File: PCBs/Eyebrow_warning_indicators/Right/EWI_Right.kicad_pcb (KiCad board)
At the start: 2 copper layers, 96.1 x 78.8 mm, 43 parts, among them J1 Conn_01x02_Female, J2 Conn_01x06_Male, J3 Conn_01x08_Male, J4 Conn_01x02_Female, J5 Conn_01x02_Female, SW1 IN SWTCH, SW2 OUT SWTCH

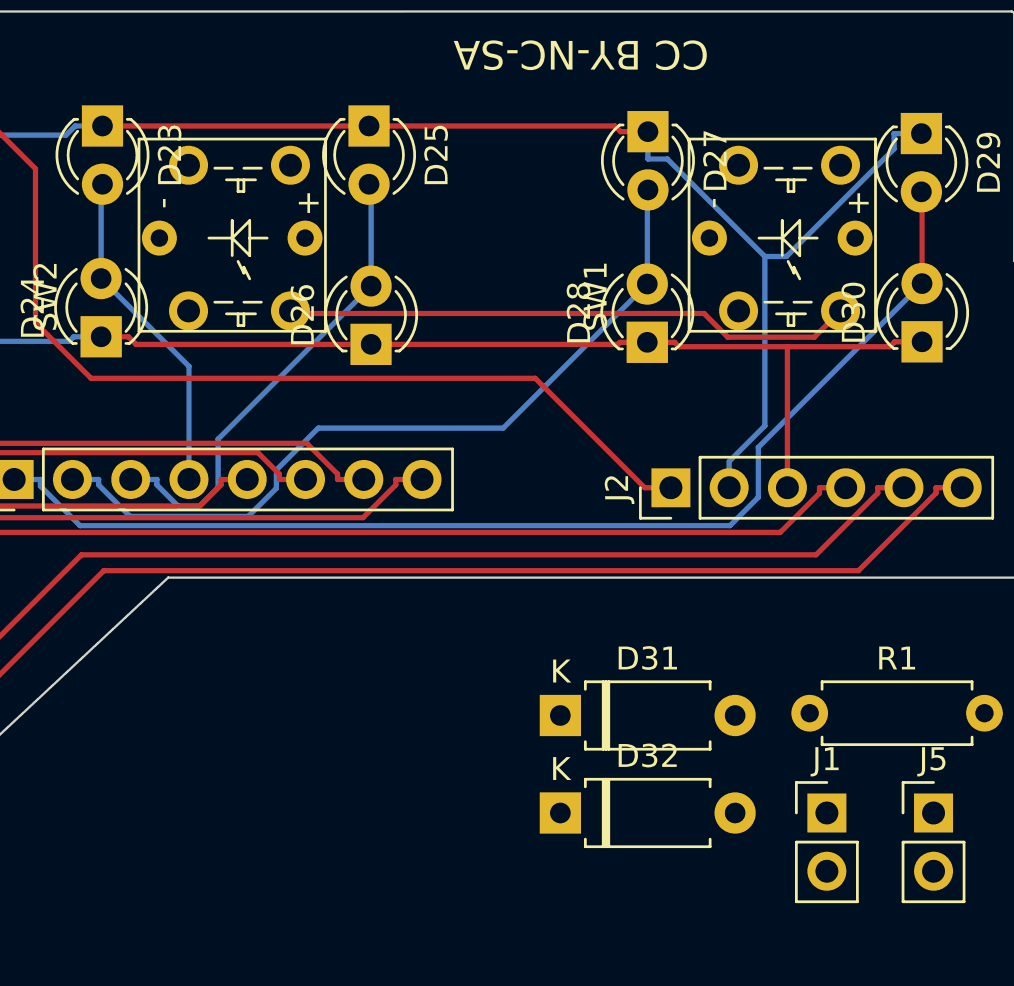
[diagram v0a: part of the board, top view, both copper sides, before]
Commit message: pcb
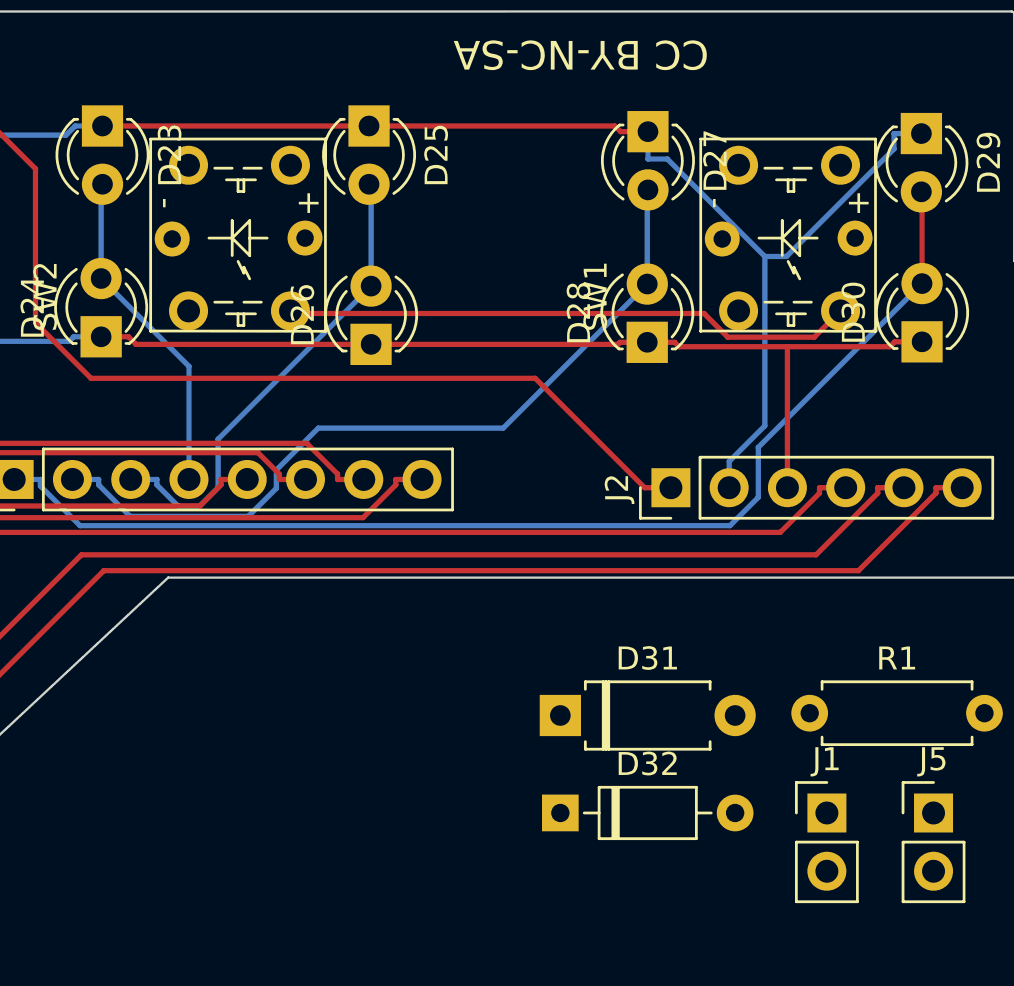
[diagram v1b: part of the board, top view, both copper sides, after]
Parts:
- D32: footprint Diode_THT:D_A-405_P7.62mm_Horizontal -> Diode_THT:D_DO-35_SOD27_P7.62mm_Horizontal
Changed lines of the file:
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@@
     (uvia_drill 0.1)
+  )
+  (module Diode_THT:D_DO-35_SOD27_P7.62mm_Horizontal (layer F.Cu)
+    (at 196.34 79.83)
+    (descr "Diode, DO-35_SOD27 series, Axial, Horizontal, pin pitch=7.62mm, , length*diameter=4*2mm^2, , http://www.diodes.com/_files/packages/DO-35.pdf")
+    (tags "Diode DO-35_SOD27 series Axial Horizontal pin pitch 7.62mm  length 4mm diameter 2mm")
+    (fp_text reference D32 (at 3.81 -2.12) (layer F.SilkS)
+      (effects (font (size 1 1) (thickness 0.15)))
+    )
+    (fp_text value D (at 3.81 2.12) (layer F.Fab)
+      (effects (font (size 1 1) (thickness 0.15)))
+    )
+    (fp_text user K (at 0 -1.8) (layer F.Fab)
+      (effects (font (size 1 1) (thickness 0.15)))
+    )
+    (fp_text user K (at 0 -1.8) (layer F.Fab)
+      (effects (font (size 1 1) (thickness 0.15)))
+    )
+    (fp_text user %R (at 4.11 0) (layer F.Fab)
+      (effects (font (size 0.8 0.8) (thickness 0.12)))
+    )
+    (fp_line (start 8.67 -1.25) (end -1.05 -1.25) (layer F.CrtYd) (width 0.05))
+    (fp_line (start 8.67 1.25) (end 8.67 -1.25) (layer F.CrtYd) (width 0.05))
+    (fp_line (start -1.05 1.25) (end 8.67 1.25) (layer F.CrtYd) (width 0.05))
+    (fp_line (start -1.05 -1.25) (end -1.05 1.25) (layer F.CrtYd) (width 0.05))
+    (fp_line (start 2.29 -1.12) (end 2.29 1.12) (layer F.SilkS) (width 0.12))
+    (fp_line (start 2.53 -1.12) (end 2.53 1.12) (layer F.SilkS) (width 0.12))
+    (fp_line (start 2.41 -1.12) (end 2.41 1.12) (layer F.SilkS) (width 0.12))
+    (fp_line (start 6.58 0) (end 5.93 0) (layer F.SilkS) (width 0.12))
+    (fp_line (start 1.04 0) (end 1.69 0) (layer F.SilkS) (width 0.12))
+    (fp_line (start 5.93 -1.12) (end 1.69 -1.12) (layer F.SilkS) (width 0.12))
+    (fp_line (start 5.93 1.12) (end 5.93 -1.12) (layer F.SilkS) (width 0.12))
+    (fp_line (start 1.69 1.12) (end 5.93 1.12) (layer F.SilkS) (width 0.12))
+    (fp_line (start 1.69 -1.12) (end 1.69 1.12) (layer F.SilkS) (width 0.12))
+    (fp_line (start 2.31 -1) (end 2.31 1) (layer F.Fab) (width 0.1))
+    (fp_line (start 2.51 -1) (end 2.51 1) (layer F.Fab) (width 0.1))
+    (fp_line (start 2.41 -1) (end 2.41 1) (layer F.Fab) (width 0.1))
+    (fp_line (start 7.62 0) (end 5.81 0) (layer F.Fab) (width 0.1))
+    (fp_line (start 0 0) (end 1.81 0) (layer F.Fab) (width 0.1))
+    (fp_line (start 5.81 -1) (end 1.81 -1) (layer F.Fab) (width 0.1))
+    (fp_line (start 5.81 1) (end 5.81 -1) (layer F.Fab) (width 0.1))
+    (fp_line (start 1.81 1) (end 5.81 1) (layer F.Fab) (width 0.1))
+    (fp_line (start 1.81 -1) (end 1.81 1) (layer F.Fab) (width 0.1))
+    (pad 2 thru_hole oval (at 7.62 0) (size 1.6 1.6) (drill 0.8) (layers *.Cu *.Mask)
+      (net 17 "Net-(D32-Pad2)"))
+    (pad 1 thru_hole rect (at 0 0) (size 1.6 1.6) (drill 0.8) (layers *.Cu *.Mask)
+      (net 18 "Net-(D32-Pad1)"))
+    (model ${KISYS3DMOD}/Diode_THT.3dshapes/D_DO-35_SOD27_P7.62mm_Horizontal.wrl
+      (at (xyz 0 0 0))
+      (scale (xyz 1 1 1))
+      (rotate (xyz 0 0 0))
+    )
   )
   (module Resistor_THT:R_Axial_DIN0207_L6.3mm_D2.5mm_P7.62mm_Horizontal (layer F.Cu)
@@
   )
   (module Diode_THT:D_A-405_P7.62mm_Horizontal (layer F.Cu)
-    (at 196.34 79.83)
-    (descr "Diode, A-405 series, Axial, Horizontal, pin pitch=7.62mm, , length*diameter=5.2*2.7mm^2, , http://www.diodes.com/_files/packages/A-405.pdf")
-    (tags "Diode A-405 series Axial Horizontal pin pitch 7.62mm  length 5.2mm diameter 2.7mm")
-    (fp_text reference D32 (at 3.81 -2.47) (layer F.SilkS)
-      (effects (font (size 1 1) (thickness 0.15)))
-    )
-    (fp_text value D (at 3.81 2.47) (layer F.Fab)
-      (effects (font (size 1 1) (thickness 0.15)))
-    )
-    (fp_text user K (at 0 -1.9) (layer F.SilkS)
-      (effects (font (size 1 1) (thickness 0.15)))
-    )
-    (fp_text user K (at 0 -1.9) (layer F.Fab)
-      (effects (font (size 1 1) (thickness 0.15)))
-    )
-    (fp_text user %R (at 4.2 0) (layer F.Fab)
-      (effects (font (size 1 1) (thickness 0.15)))
-    )
-    (fp_line (start 8.77 -1.6) (end -1.15 -1.6) (layer F.CrtYd) (width 0.05))
-    (fp_line (start 8.77 1.6) (end 8.77 -1.6) (layer F.CrtYd) (width 0.05))
-    (fp_line (start -1.15 1.6) (end 8.77 1.6) (layer F.CrtYd) (width 0.05))
-    (fp_line (start -1.15 -1.6) (end -1.15 1.6) (layer F.CrtYd) (width 0.05))
-    (fp_line (start 1.87 -1.47) (end 1.87 1.47) (layer F.SilkS) (width 0.12))
-    (fp_line (start 2.11 -1.47) (end 2.11 1.47) (layer F.SilkS) (width 0.12))
-    (fp_line (start 1.99 -1.47) (end 1.99 1.47) (layer F.SilkS) (width 0.12))
-    (fp_line (start 6.53 1.47) (end 6.53 1.14) (layer F.SilkS) (width 0.12))
-    (fp_line (start 1.09 1.47) (end 6.53 1.47) (layer F.SilkS) (width 0.12))
-    (fp_line (start 1.09 1.14) (end 1.09 1.47) (layer F.SilkS) (width 0.12))
-    (fp_line (start 6.53 -1.47) (end 6.53 -1.14) (layer F.SilkS) (width 0.12))
-    (fp_line (start 1.09 -1.47) (end 6.53 -1.47) (layer F.SilkS) (width 0.12))
-    (fp_line (start 1.09 -1.14) (end 1.09 -1.47) (layer F.SilkS) (width 0.12))
-    (fp_line (start 1.89 -1.35) (end 1.89 1.35) (layer F.Fab) (width 0.1))
-    (fp_line (start 2.09 -1.35) (end 2.09 1.35) (layer F.Fab) (width 0.1))
-    (fp_line (start 1.99 -1.35) (end 1.99 1.35) (layer F.Fab) (width 0.1))
-    (fp_line (start 7.62 0) (end 6.41 0) (layer F.Fab) (width 0.1))
-    (fp_line (start 0 0) (end 1.21 0) (layer F.Fab) (width 0.1))
-    (fp_line (start 6.41 -1.35) (end 1.21 -1.35) (layer F.Fab) (width 0.1))
-    (fp_line (start 6.41 1.35) (end 6.41 -1.35) (layer F.Fab) (width 0.1))
-    (fp_line (start 1.21 1.35) (end 6.41 1.35) (layer F.Fab) (width 0.1))
-    (fp_line (start 1.21 -1.35) (end 1.21 1.35) (layer F.Fab) (width 0.1))
-    (pad 2 thru_hole oval (at 7.62 0) (size 1.8 1.8) (drill 0.9) (layers *.Cu *.Mask)
-      (net 17 "Net-(D32-Pad2)"))
-    (pad 1 thru_hole rect (at 0 0) (size 1.8 1.8) (drill 0.9) (layers *.Cu *.Mask)
-      (net 18 "Net-(D32-Pad1)"))
-    (model ${KISYS3DMOD}/Diode_THT.3dshapes/D_A-405_P7.62mm_Horizontal.wrl
-      (at (xyz 0 0 0))
-      (scale (xyz 1 1 1))
-      (rotate (xyz 0 0 0))
-    )
-  )
-  (module Diode_THT:D_A-405_P7.62mm_Horizontal (layer F.Cu)
     (at 196.34 75.58)
     (descr "Diode, A-405 series, Axial, Horizontal, pin pitch=7.62mm, , length*diameter=5.2*2.7mm^2, , http://www.diodes.com/_files/packages/A-405.pdf")
@@
       (effects (font (size 1 1) (thickness 0.15)))
     )
-    (fp_text user K (at 0 -1.9) (layer F.SilkS)
+    (fp_text user K (at 0 -1.9) (layer F.Fab)
       (effects (font (size 1 1) (thickness 0.15)))
     )
@@
     )
     (fp_line (start -4.318 -3.81) (end -3.048 -3.81) (layer F.SilkS) (width 0.12))
-    (fp_line (start -4.318 4.318) (end -4.318 -3.81) (layer F.SilkS) (width 0.12))
-    (fp_line (start 4.064 4.318) (end -4.318 4.318) (layer F.SilkS) (width 0.12))
-    (fp_line (start 4.064 -3.81) (end 4.064 4.318) (layer F.SilkS) (width 0.12))
+    (fp_line (start -4.32 3.81) (end -4.318 -3.81) (layer F.SilkS) (width 0.12))
+    (fp_line (start 4.07 3.81) (end -4.312 3.81) (layer F.SilkS) (width 0.12))
+    (fp_line (start 4.064 -3.81) (end 4.05 3.81) (layer F.SilkS) (width 0.12))
     (fp_line (start -4.064 -3.81) (end 4.064 -3.81) (layer F.SilkS) (width 0.12))
     (fp_text user - (at -1.524 3.302 90) (layer F.SilkS)
@@
       (effects (font (size 1 1) (thickness 0.15)))
     )
-    (pad 6 thru_hole circle (at 0 3.429 270) (size 1.524 1.524) (drill 0.762) (layers *.Cu *.Mask)
+    (pad 6 thru_hole circle (at 0.04 2.87 270) (size 1.524 1.524) (drill 0.762) (layers *.Cu *.Mask)
       (net 19 "Net-(J1-Pad2)"))
     (pad 5 thru_hole circle (at 0 -2.921 270) (size 1.524 1.524) (drill 0.762) (layers *.Cu *.Mask)
@@
     )
     (fp_line (start -4.318 -3.81) (end -3.048 -3.81) (layer F.SilkS) (width 0.12))
-    (fp_line (start -4.318 4.318) (end -4.318 -3.81) (layer F.SilkS) (width 0.12))
-    (fp_line (start 4.064 4.318) (end -4.318 4.318) (layer F.SilkS) (width 0.12))
-    (fp_line (start 4.064 -3.81) (end 4.064 4.318) (layer F.SilkS) (width 0.12))
+    (fp_line (start -4.32 3.81) (end -4.318 -3.81) (layer F.SilkS) (width 0.12))
+    (fp_line (start 4.07 3.81) (end -4.312 3.81) (layer F.SilkS) (width 0.12))
+    (fp_line (start 4.064 -3.81) (end 4.05 3.81) (layer F.SilkS) (width 0.12))
     (fp_line (start -4.064 -3.81) (end 4.064 -3.81) (layer F.SilkS) (width 0.12))
     (fp_text user - (at -1.524 3.302 90) (layer F.SilkS)
@@
       (effects (font (size 1 1) (thickness 0.15)))
     )
-    (pad 6 thru_hole circle (at 0 3.429 270) (size 1.524 1.524) (drill 0.762) (layers *.Cu *.Mask)
+    (pad 6 thru_hole circle (at 0.04 2.87 270) (size 1.524 1.524) (drill 0.762) (layers *.Cu *.Mask)
       (net 24 "Net-(SW1-Pad6)"))
     (pad 5 thru_hole circle (at 0 -2.921 270) (size 1.524 1.524) (drill 0.762) (layers *.Cu *.Mask)
